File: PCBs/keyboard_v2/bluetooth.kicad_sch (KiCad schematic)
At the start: 19 parts, among them U1001 nRF52840-QFAA-F-R7, Y1002 32MHz

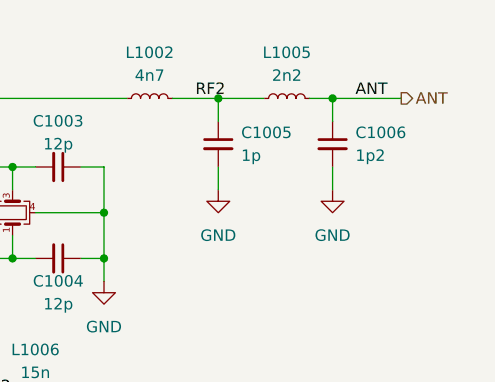
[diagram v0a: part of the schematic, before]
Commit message: Layout in progress
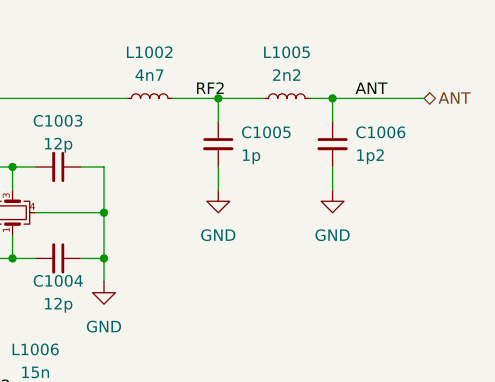
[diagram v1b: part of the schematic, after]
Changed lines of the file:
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@@
 	(wire
 		(pts
-			(xy 200.66 53.34) (xy 208.28 53.34)
+			(xy 200.66 53.34) (xy 210.82 53.34)
 		)
 		(stroke
@@
 			)
 			(justify left bottom)
-		)
-	)
-	(hierarchical_label "ANT"
-		(shape output)
-		(at 208.28 53.34 0)
-		(fields_autoplaced yes)
-		(effects
-			(font
-				(size 1.27 1.27)
-			)
-			(justify left)
 		)
 	)
@@
 		)
 	)
+	(hierarchical_label "ANT"
+		(shape bidirectional)
+		(at 210.82 53.34 0)
+		(fields_autoplaced yes)
+		(effects
+			(font
+				(size 1.27 1.27)
+			)
+			(justify left)
+		)
+	)
